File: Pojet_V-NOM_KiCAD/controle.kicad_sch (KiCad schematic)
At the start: 10 parts, among them U1 STM32G431CBU6, Y1 Crystal_GND24_Small

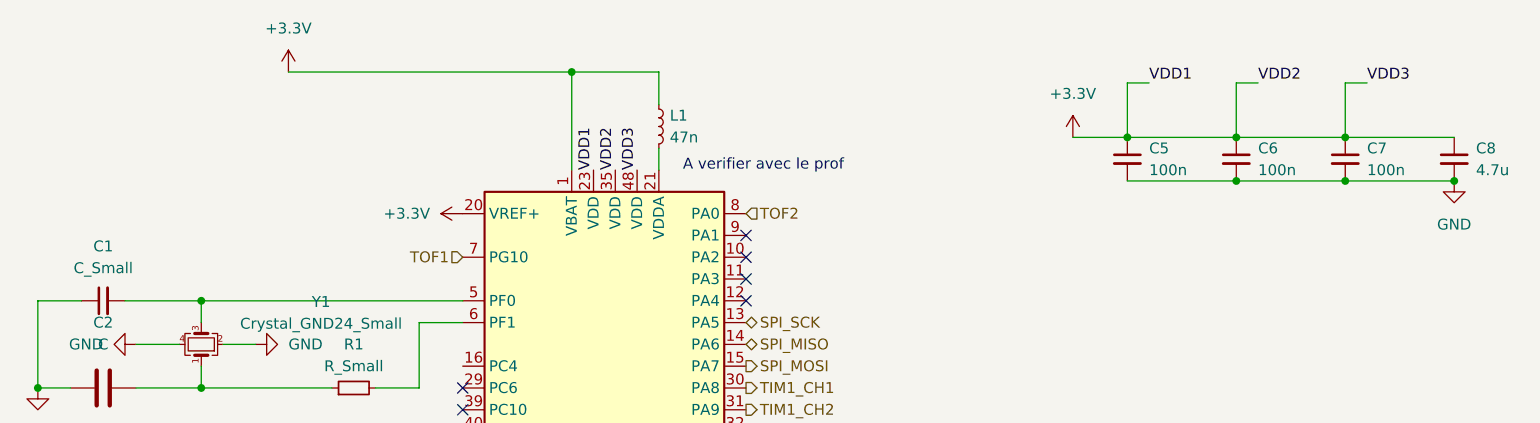
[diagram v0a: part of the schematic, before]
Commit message: Mise à jour du schéma de contrôle
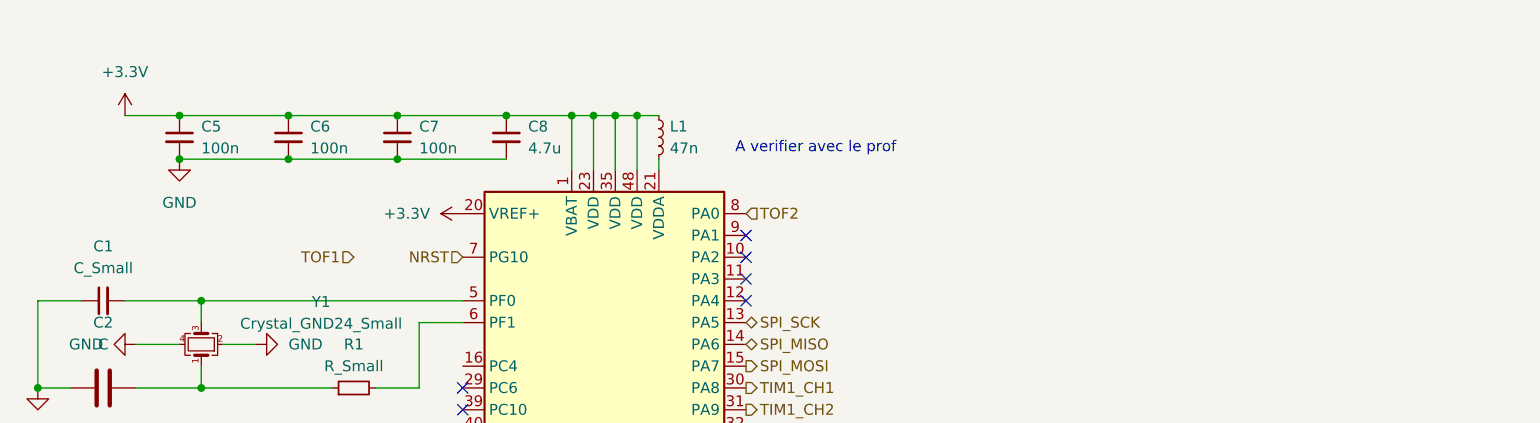
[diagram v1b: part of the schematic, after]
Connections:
- net TOF1: no longer U1.7 (PG10)
- new net NRST: U1.7 (PG10)
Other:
- moved on the sheet: C5, C6, C7, C8, L1
